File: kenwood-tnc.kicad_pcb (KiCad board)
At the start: 2 copper layers, 58.4 x 33.7 mm, 12 parts, among them J1 DB9_Female, J2 PC Speaker, J3 PC MIC, J4 Radio MIC, J5 Radio Speaker, Q1 BC547C

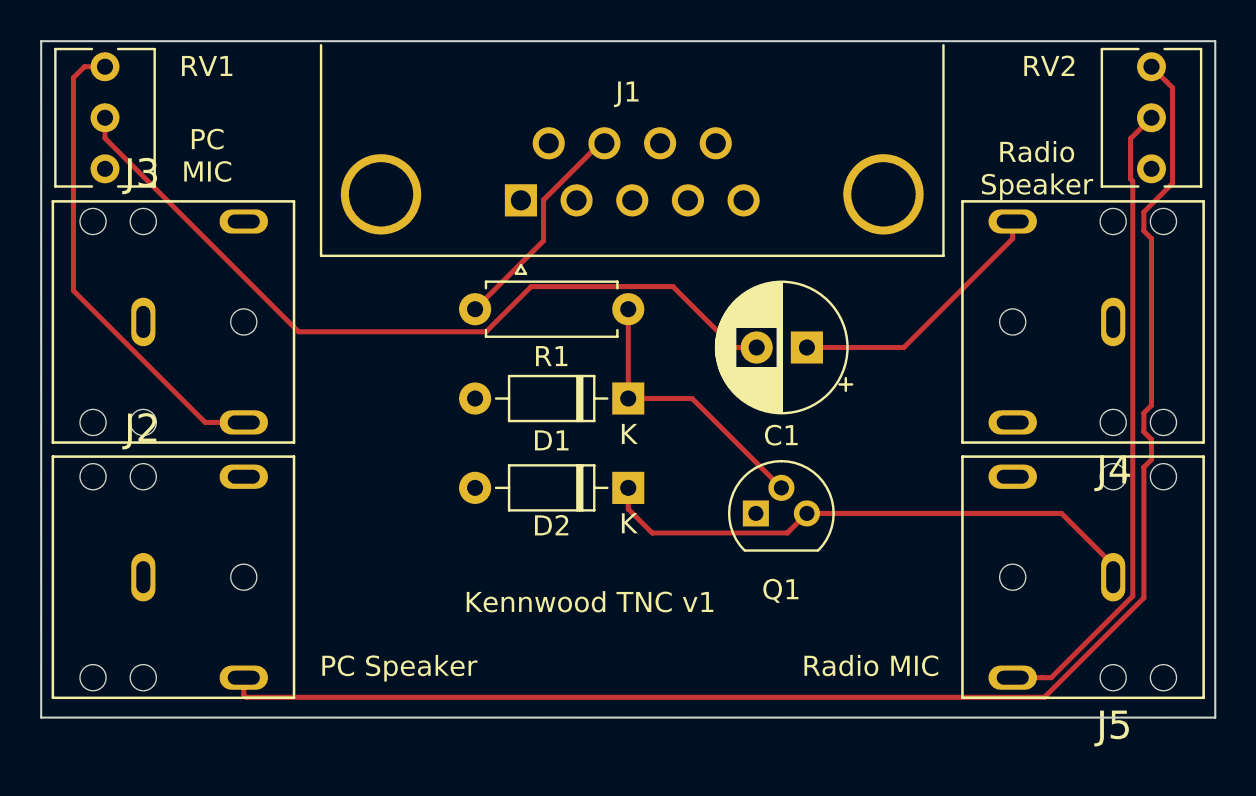
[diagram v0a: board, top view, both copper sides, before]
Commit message: KiCAD update
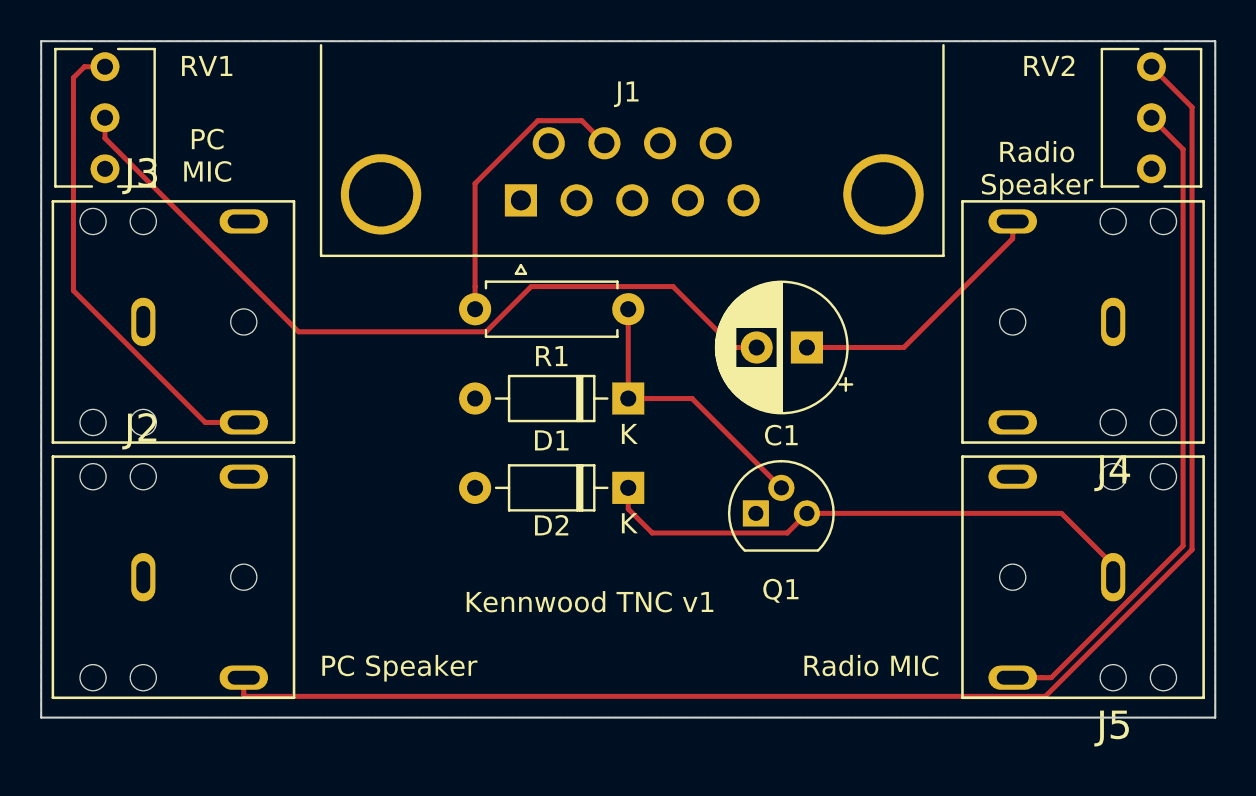
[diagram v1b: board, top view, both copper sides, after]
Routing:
- net Net-(J1-Pad7): track 11.0 -> 14.7 mm
- net Net-(J5-Pad2): track 31.9 -> 33.1 mm
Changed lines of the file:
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@@
     (thickness 1.6)
     (drawings 9)
-    (tracks 55)
+    (tracks 42)
     (zones 0)
     (modules 12)
@@
     (effects (font (size 1 1) (thickness 0.15)))
   )
-  (segment (start 95.33 30.144) (end 95.33 29.29) (width 0.25) (layer F.Cu) (net 1))
+  (segment (start 95.33 30.144) (end 95.33 29.29) (width 0.25) (layer F.Cu) (net 1) (status 20))
   (segment (start 89.914 35.56) (end 95.33 30.144) (width 0.25) (layer F.Cu) (net 1))
-  (segment (start 85.09 35.56) (end 89.914 35.56) (width 0.25) (layer F.Cu) (net 1))
+  (segment (start 85.09 35.56) (end 89.914 35.56) (width 0.25) (layer F.Cu) (net 1) (status 10))
   (segment (start 59.796768 34.780001) (end 50.165 25.148233) (width 0.25) (layer F.Cu) (net 2))
   (segment (start 71.370003 32.529999) (end 69.120001 34.780001) (width 0.25) (layer F.Cu) (net 2))
   (segment (start 78.428629 32.529999) (end 71.370003 32.529999) (width 0.25) (layer F.Cu) (net 2))
-  (segment (start 50.165 25.148233) (end 50.165 24.13) (width 0.25) (layer F.Cu) (net 2))
+  (segment (start 50.165 25.148233) (end 50.165 24.13) (width 0.25) (layer F.Cu) (net 2) (status 20))
   (segment (start 81.45863 35.56) (end 78.428629 32.529999) (width 0.25) (layer F.Cu) (net 2))
   (segment (start 69.120001 34.780001) (end 59.796768 34.780001) (width 0.25) (layer F.Cu) (net 2))
-  (segment (start 82.59 35.56) (end 81.45863 35.56) (width 0.25) (layer F.Cu) (net 2))
+  (segment (start 82.59 35.56) (end 81.45863 35.56) (width 0.25) (layer F.Cu) (net 2) (status 10))
   (segment (start 76.2 38.1) (end 76.2 33.655) (width 0.25) (layer F.Cu) (net 4) (status 30))
   (segment (start 79.375 38.1) (end 83.82 42.545) (width 0.25) (layer F.Cu) (net 4) (status 20))
@@
   (segment (start 76.2 43.595) (end 77.395001 44.790001) (width 0.25) (layer F.Cu) (net 5))
   (segment (start 76.2 42.545) (end 76.2 43.595) (width 0.25) (layer F.Cu) (net 5) (status 10))
-  (segment (start 86.009238 43.815) (end 85.09 43.815) (width 0.25) (layer F.Cu) (net 5))
-  (segment (start 97.759 43.815) (end 86.009238 43.815) (width 0.25) (layer F.Cu) (net 5))
-  (segment (start 100.33 46.386) (end 97.759 43.815) (width 0.25) (layer F.Cu) (net 5))
-  (segment (start 100.33 46.99) (end 100.33 46.386) (width 0.25) (layer F.Cu) (net 5))
-  (segment (start 71.985001 30.249999) (end 68.58 33.655) (width 0.25) (layer F.Cu) (net 11) (status 20))
-  (segment (start 71.985001 28.219997) (end 71.985001 30.249999) (width 0.25) (layer F.Cu) (net 11))
-  (segment (start 74.804998 25.4) (end 71.985001 28.219997) (width 0.25) (layer F.Cu) (net 11) (status 10))
+  (segment (start 97.759 43.815) (end 85.09 43.815) (width 0.25) (layer F.Cu) (net 5) (status 20))
+  (segment (start 100.33 46.386) (end 97.759 43.815) (width 0.25) (layer F.Cu) (net 5) (status 10))
+  (segment (start 100.33 46.99) (end 100.33 46.386) (width 0.25) (layer F.Cu) (net 5) (status 30))
   (segment (start 75.015 25.4) (end 74.804998 25.4) (width 0.25) (layer F.Cu) (net 11) (status 30))
-  (segment (start 102.954999 22.309999) (end 102.235 21.59) (width 0.25) (layer F.Cu) (net 15))
-  (segment (start 103.280001 22.635001) (end 102.954999 22.309999) (width 0.25) (layer F.Cu) (net 15))
-  (segment (start 103.280001 27.396997) (end 103.280001 22.635001) (width 0.25) (layer F.Cu) (net 15))
-  (segment (start 101.854999 28.821999) (end 103.280001 27.396997) (width 0.25) (layer F.Cu) (net 15))
-  (segment (start 101.854999 29.758001) (end 101.854999 28.821999) (width 0.25) (layer F.Cu) (net 15))
-  (segment (start 102.235 38.441998) (end 102.235 30.138002) (width 0.25) (layer F.Cu) (net 15))
-  (segment (start 101.854999 38.821999) (end 102.235 38.441998) (width 0.25) (layer F.Cu) (net 15))
-  (segment (start 101.854999 39.758001) (end 101.854999 38.821999) (width 0.25) (layer F.Cu) (net 15))
-  (segment (start 101.854999 41.521999) (end 102.235 41.141998) (width 0.25) (layer F.Cu) (net 15))
-  (segment (start 101.854999 48.019229) (end 101.854999 41.521999) (width 0.25) (layer F.Cu) (net 15))
-  (segment (start 96.909227 52.965001) (end 101.854999 48.019229) (width 0.25) (layer F.Cu) (net 15))
-  (segment (start 102.235 30.138002) (end 101.854999 29.758001) (width 0.25) (layer F.Cu) (net 15))
-  (segment (start 57.191001 52.965001) (end 96.909227 52.965001) (width 0.25) (layer F.Cu) (net 15))
-  (segment (start 102.235 41.141998) (end 102.235 40.138002) (width 0.25) (layer F.Cu) (net 15))
-  (segment (start 57.07 52.844) (end 57.191001 52.965001) (width 0.25) (layer F.Cu) (net 15))
-  (segment (start 102.235 40.138002) (end 101.854999 39.758001) (width 0.25) (layer F.Cu) (net 15))
-  (segment (start 57.07 51.99) (end 57.07 52.844) (width 0.25) (layer F.Cu) (net 15))
-  (segment (start 55.612 39.29) (end 57.07 39.29) (width 0.25) (layer F.Cu) (net 17))
-  (segment (start 55.152182 39.29) (end 55.612 39.29) (width 0.25) (layer F.Cu) (net 17))
+  (segment (start 68.58 32.52363) (end 68.58 33.655) (width 0.25) (layer F.Cu) (net 11))
+  (segment (start 68.58 27.399998) (end 68.58 32.52363) (width 0.25) (layer F.Cu) (net 11))
+  (segment (start 73.889999 24.274999) (end 71.704999 24.274999) (width 0.25) (layer F.Cu) (net 11))
+  (segment (start 71.704999 24.274999) (end 68.58 27.399998) (width 0.25) (layer F.Cu) (net 11))
+  (segment (start 75.015 25.4) (end 73.889999 24.274999) (width 0.25) (layer F.Cu) (net 11))
+  (segment (start 57.07 52.844) (end 57.07 51.99) (width 0.25) (layer F.Cu) (net 15))
+  (segment (start 57.14501 52.91901) (end 57.07 52.844) (width 0.25) (layer F.Cu) (net 15))
+  (segment (start 96.955218 52.91901) (end 57.14501 52.91901) (width 0.25) (layer F.Cu) (net 15))
+  (segment (start 104.25501 45.619218) (end 96.955218 52.91901) (width 0.25) (layer F.Cu) (net 15))
+  (segment (start 104.255011 23.610011) (end 104.25501 45.619218) (width 0.25) (layer F.Cu) (net 15))
+  (segment (start 102.235 21.59) (end 104.255011 23.610011) (width 0.25) (layer F.Cu) (net 15))
+  (segment (start 55.152182 39.29) (end 57.07 39.29) (width 0.25) (layer F.Cu) (net 17) (status 20))
   (segment (start 48.594999 32.732817) (end 55.152182 39.29) (width 0.25) (layer F.Cu) (net 17))
   (segment (start 48.594999 22.141768) (end 48.594999 32.732817) (width 0.25) (layer F.Cu) (net 17))
   (segment (start 49.146767 21.59) (end 48.594999 22.141768) (width 0.25) (layer F.Cu) (net 17))
-  (segment (start 50.165 21.59) (end 49.146767 21.59) (width 0.25) (layer F.Cu) (net 17))
+  (segment (start 50.165 21.59) (end 49.146767 21.59) (width 0.25) (layer F.Cu) (net 17) (status 10))
   (segment (start 96.788 51.99) (end 95.33 51.99) (width 0.25) (layer F.Cu) (net 19))
+  (segment (start 103.805001 25.700001) (end 103.805001 45.432817) (width 0.25) (layer F.Cu) (net 19))
   (segment (start 97.247818 51.99) (end 96.788 51.99) (width 0.25) (layer F.Cu) (net 19))
-  (segment (start 101.305001 47.932817) (end 97.247818 51.99) (width 0.25) (layer F.Cu) (net 19))
-  (segment (start 101.305001 27.286603) (end 101.305001 47.932817) (width 0.25) (layer F.Cu) (net 19))
-  (segment (start 101.189999 27.171601) (end 101.305001 27.286603) (width 0.25) (layer F.Cu) (net 19))
-  (segment (start 101.189999 25.175001) (end 101.189999 27.171601) (width 0.25) (layer F.Cu) (net 19))
-  (segment (start 102.235 24.13) (end 101.189999 25.175001) (width 0.25) (layer F.Cu) (net 19))
+  (segment (start 103.805001 45.432817) (end 97.247818 51.99) (width 0.25) (layer F.Cu) (net 19))
+  (segment (start 102.235 24.13) (end 103.805001 25.700001) (width 0.25) (layer F.Cu) (net 19))
   (zone (net 3) (net_name GND) (layer B.Cu) (hatch edge 0.508)
     (connect_pads (clearance 0.508))
